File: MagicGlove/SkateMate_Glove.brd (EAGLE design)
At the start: 40 x 23.3 mm, 41 parts, among them U1 ATMEGA328P-AU, Y1 8MHz

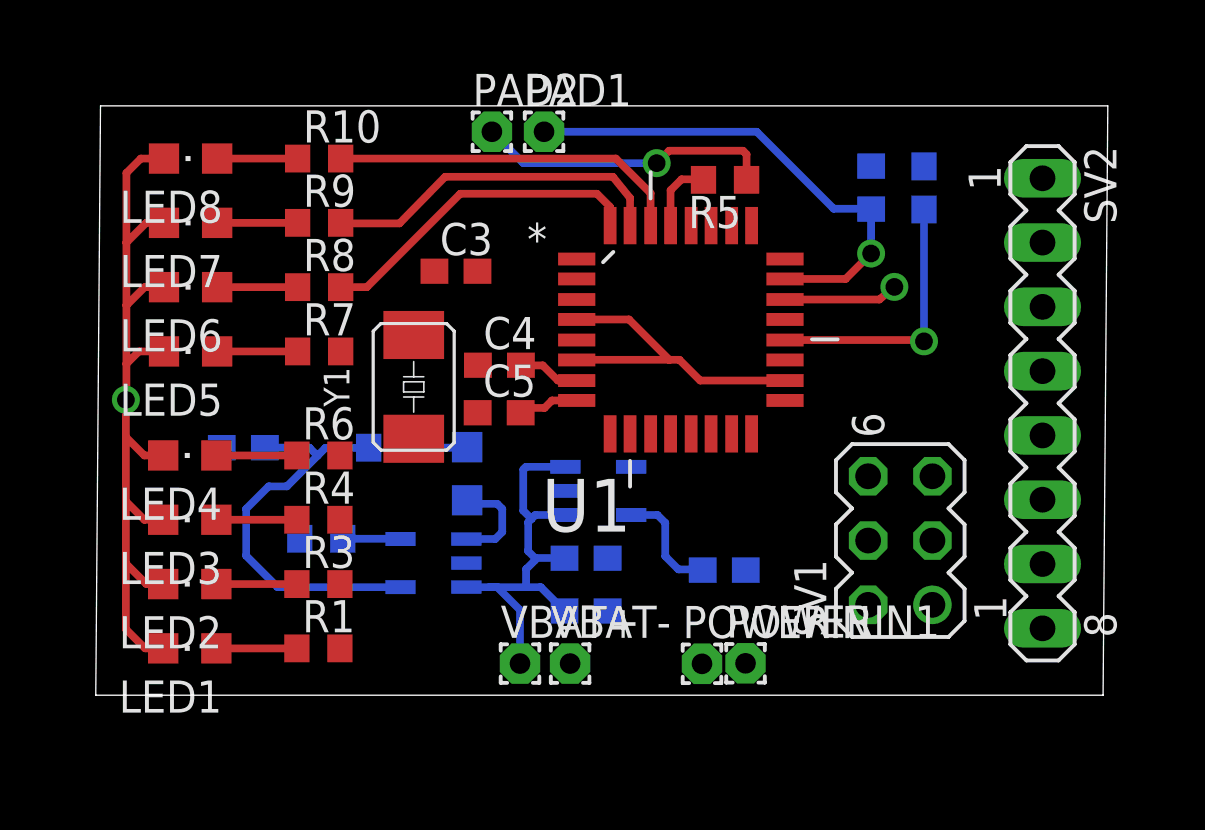
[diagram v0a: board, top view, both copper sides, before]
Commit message: Version 0.1 Layout
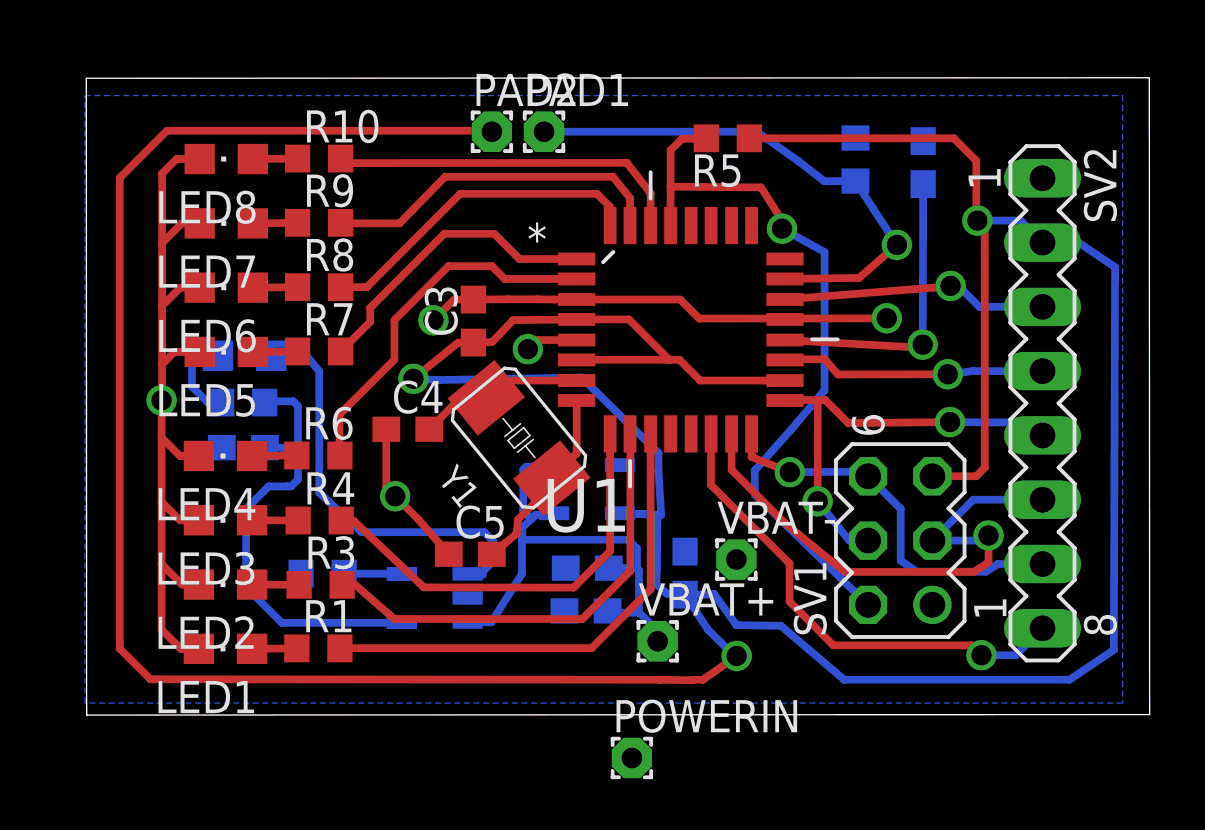
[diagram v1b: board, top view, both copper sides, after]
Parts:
- removed POWERIN1: -, wirepad:1,6/0,8
- IC1: value (none) -> BU33TD3WG
- moved LED9 9.95 mm to (5.31, 12.7), turned to 90 degrees
- moved VBAT- 7.75 mm to (24.7, 4.67)
- moved R12 6.08 mm to (5.25, 10.9), turned to 0 degrees
- moved C5 5.71 mm to (14.2, 4.88)
- moved VBAT+ 5.51 mm to (21.6, 1.44)
- moved POWERIN 4.64 mm to (20.6, -3.17)
- moved Y1 4.62 mm to (16.2, 9.47), turned to 129.2 degrees
- moved C4 4.42 mm to (11.8, 9.82)
- moved C3 2.09 mm to (14.3, 14.1), turned to 90 degrees
- moved R5 1.64 mm to (24.4, 21.3)
- moved C7 1.55 mm to (22.7, 4.13), turned to 90 degrees
- moved LED5 1.41 mm to (4.58, 12.9)
- moved LED6 1.41 mm to (4.58, 15.4)
- moved LED7 1.41 mm to (4.58, 18.0)
- moved LED8 1.41 mm to (4.58, 20.5)
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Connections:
- net GND: no longer POWERIN1.1, Y1.P$1, Y1.P$2
- net N$3: now also Y1.P$1
- net N$4: now also Y1.P$2
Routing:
- net +3V3: track 29.2 -> 167.0 mm, vias 1 -> 3
- net GND: track 32.2 -> 58.9 mm, vias 1 -> 5
- net RESETICSP: track 2.88 -> 28.8 mm, vias 0 -> 1
- net MOSI: track 0.00 -> 21.6 mm, vias 0 -> 1
- net N$12: track 0.00 -> 19.4 mm
- net IRQ: track 0.00 -> 19.2 mm, vias 0 -> 1
- net N$13: track 0.00 -> 18.1 mm
- net SCK: track 0.00 -> 17.4 mm, vias 0 -> 2
- net N$15: track 0.00 -> 16.9 mm
- net MISO: track 0.00 -> 15.4 mm, vias 0 -> 1
- net N$16: track 0.00 -> 14.5 mm
- net N$23: track 3.98 -> 17.2 mm
- net N$17: track 0.00 -> 12.0 mm
- net CSN: track 0.00 -> 10.5 mm, vias 0 -> 1
- net CE: track 4.50 -> 10.5 mm
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- added copper zone on layer 16, net GND
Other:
- board size 40 x 23.3 mm -> 42 x 25.2 mm

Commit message: V0.9 Layout and Schematic ready for review and version jump to 1.0.
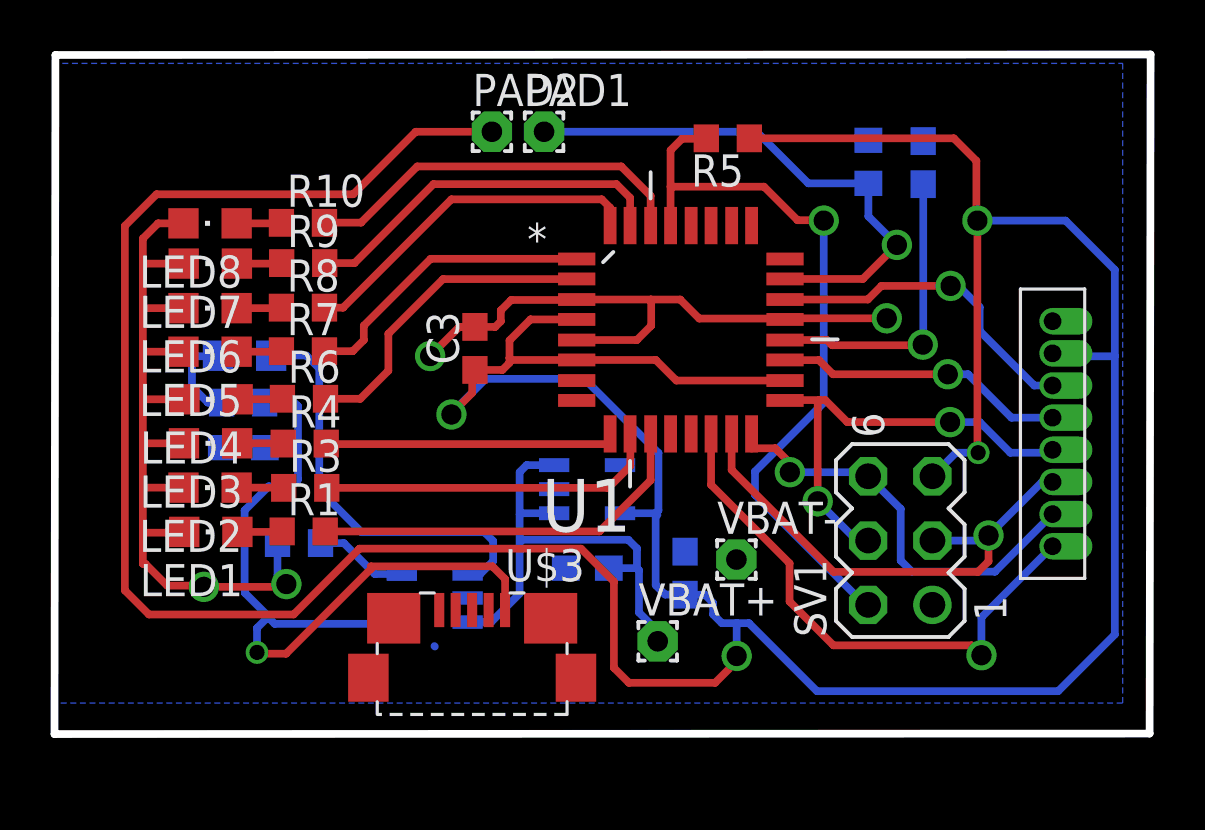
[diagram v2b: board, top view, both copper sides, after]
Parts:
- removed C10: 4.7u, eagle-ltspice:C0603
- removed C4, C5: 22p, eagle-ltspice:C0603
- removed POWERIN: +, wirepad:1,6/0,8
- removed SV2: RFM75, con-lstb:MA08-1
- removed Y1: 8MHz, crystals:ABM3
- added U$2: HEADER1,27, SkateMateMagicGlove:HEADER1,27
- added U$3: MICRO-USB-ZX62R-B-5P, con-hirose:ZX62R-B-5P
- moved LED1 4.66 mm to (3.98, 5.76)
- moved R1 4.66 mm to (7.64, 5.78)
- moved R3 3.88 mm to (7.71, 7.50)
- moved LED2 3.88 mm to (3.94, 7.51)
- moved LED3 3.10 mm to (3.96, 9.26)
- moved R4 3.10 mm to (7.68, 9.25)
- moved R10 2.62 mm to (7.62, 18.0)
- moved LED8 2.62 mm to (3.94, 18.0)
- moved LED4 2.31 mm to (3.98, 11.0)
- moved R6 2.31 mm to (7.66, 11.0)
- moved R9 1.71 mm to (7.62, 16.4)
- moved LED7 1.71 mm to (3.96, 16.4)
- moved R11 1.53 mm to (7.46, 5.32)
- moved C3 1.08 mm to (14.4, 13.0)
- moved R8 1.03 mm to (7.62, 14.6)
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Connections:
- removed net N$3: C5.2, U1.8, Y1.P$1
- removed net N$4: C4.2, U1.7, Y1.P$2
- net +3V3: now also U$2.P$2; no longer SV2.2
- net CE: now also U$2.P$3; no longer SV2.3
- net CSN: now also U$2.P$4; no longer SV2.4
- net GND: now also U$2.P$1; no longer C10.2, C4.1, C5.1, SV2.1
- net IRQ: now also U$2.P$8; no longer SV2.8
- net MISO: now also U$2.P$7; no longer SV2.7
- net MOSI: now also U$2.P$6; no longer SV2.6
- net N$21: no longer C10.1
- net N$24: now also U$3.1; no longer POWERIN.1
- net SCK: now also U$2.P$5; no longer SV2.5
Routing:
- net N$24: track 18.1 -> 32.7 mm, vias 0 -> 1
- net N$3: track 7.50 -> 0.00 mm
- net N$4: track 6.62 -> 0.00 mm
- net N$15: track 16.9 -> 11.6 mm
- net N$13: track 18.1 -> 13.6 mm
- net N$12: track 19.4 -> 15.5 mm
- net IRQ: track 19.2 -> 21.8 mm
- net CE: track 10.5 -> 13.0 mm
- net N$16: track 14.5 -> 12.7 mm
- net +3V3: track 167.0 -> 165.3 mm, vias 3 -> 4
- net MOSI: track 21.6 -> 20.1 mm
- net MISO: track 15.4 -> 16.8 mm
- net N$25: track 2.28 -> 3.73 mm
- net N$20: track 14.3 -> 15.5 mm
- net CSN: track 10.5 -> 11.6 mm
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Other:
- board size 42 x 25.2 mm -> 43.3 x 26.8 mm

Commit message: Revert "V0.9 Layout and Schematic ready for review and version jump to 1.0."
This reverts commit 28fefd69818988460ab9c4da467096be04e20f85.
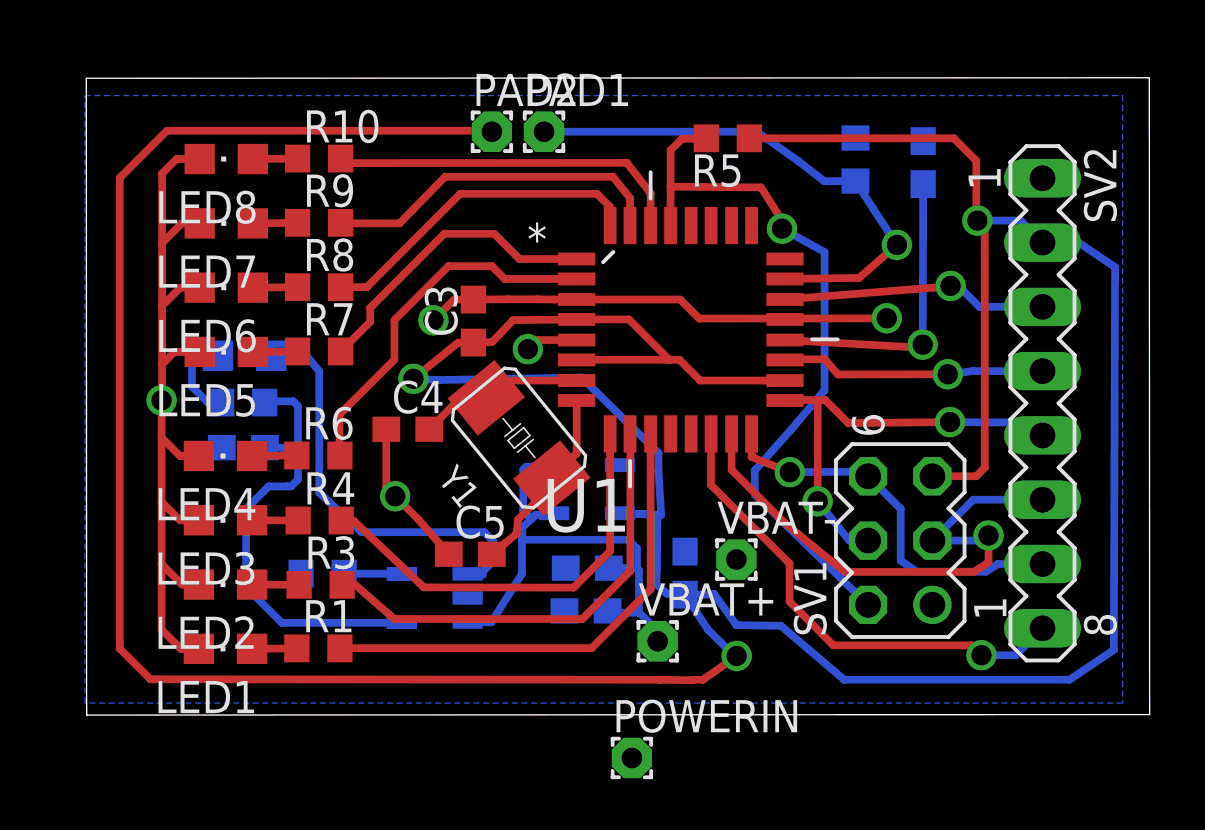
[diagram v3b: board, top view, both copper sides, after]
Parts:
- removed U$2: HEADER1,27, SkateMateMagicGlove:HEADER1,27
- removed U$3: MICRO-USB-ZX62R-B-5P, con-hirose:ZX62R-B-5P
- added C10: 4.7u, eagle-ltspice:C0603
- added C4, C5: 22p, eagle-ltspice:C0603
- added POWERIN: +, wirepad:1,6/0,8
- added SV2: RFM75, con-lstb:MA08-1
- added Y1: 8MHz, crystals:ABM3
- moved LED1 4.66 mm to (4.55, 1.14)
- moved R1 4.66 mm to (8.22, 1.16)
- moved R3 3.88 mm to (8.31, 3.67)
- moved LED2 3.88 mm to (4.55, 3.68)
- moved LED3 3.10 mm to (4.55, 6.22)
- moved R4 3.10 mm to (8.28, 6.21)
- moved R10 2.62 mm to (8.26, 20.5)
- moved LED8 2.62 mm to (4.58, 20.5)
- moved LED4 2.31 mm to (4.55, 8.76)
- moved R6 2.31 mm to (8.22, 8.78)
- moved R9 1.71 mm to (8.26, 18.0)
- moved LED7 1.71 mm to (4.58, 18.0)
- moved R11 1.53 mm to (8.39, 4.11)
- moved C3 1.08 mm to (14.3, 14.1)
- moved R8 1.03 mm to (8.26, 15.4)
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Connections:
- new net N$3: C5.2, U1.8, Y1.P$1
- new net N$4: C4.2, U1.7, Y1.P$2
- net +3V3: now also SV2.2; no longer U$2.P$2
- net CE: now also SV2.3; no longer U$2.P$3
- net CSN: now also SV2.4; no longer U$2.P$4
- net GND: now also C10.2, C4.1, C5.1, SV2.1; no longer U$2.P$1
- net IRQ: now also SV2.8; no longer U$2.P$8
- net MISO: now also SV2.7; no longer U$2.P$7
- net MOSI: now also SV2.6; no longer U$2.P$6
- net N$21: now also C10.1
- net N$24: now also POWERIN.1; no longer U$3.1
- net SCK: now also SV2.5; no longer U$2.P$5
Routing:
- net N$24: track 32.7 -> 18.1 mm, vias 1 -> 0
- net N$3: track 0.00 -> 7.50 mm
- net N$4: track 0.00 -> 6.62 mm
- net N$15: track 11.6 -> 16.9 mm
- net N$13: track 13.6 -> 18.1 mm
- net N$12: track 15.5 -> 19.4 mm
- net IRQ: track 21.8 -> 19.2 mm
- net CE: track 13.0 -> 10.5 mm
- net N$16: track 12.7 -> 14.5 mm
- net +3V3: track 165.3 -> 167.0 mm, vias 4 -> 3
- net MOSI: track 20.1 -> 21.6 mm
- net MISO: track 16.8 -> 15.4 mm
- net N$25: track 3.73 -> 2.28 mm
- net N$20: track 15.5 -> 14.3 mm
- net CSN: track 11.6 -> 10.5 mm
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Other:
- board size 43.3 x 26.8 mm -> 42 x 25.2 mm
